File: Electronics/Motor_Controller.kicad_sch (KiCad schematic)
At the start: 43 parts, among them J2 SWCLK SWD, SW1 SW_Push, SW2 ~{USB_BOOT}, U1 RP2040, U4 W25Q32JVZP, Y1 ABM8-272-T3

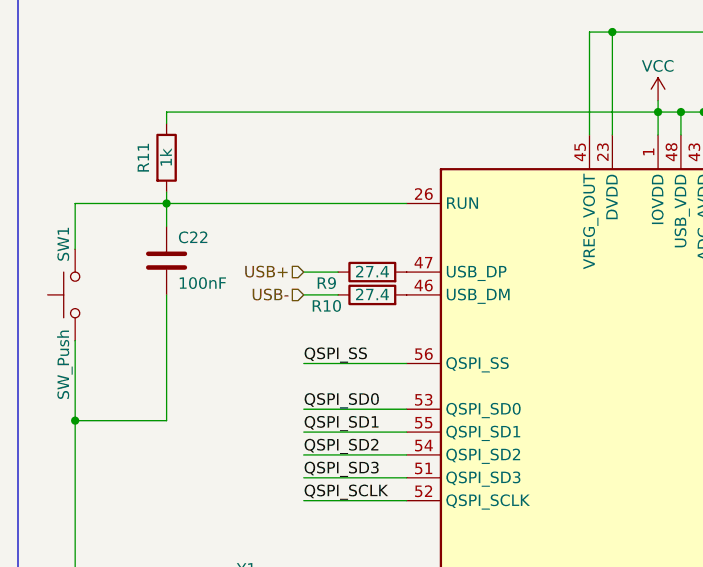
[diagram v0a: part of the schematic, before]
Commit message: power + usb
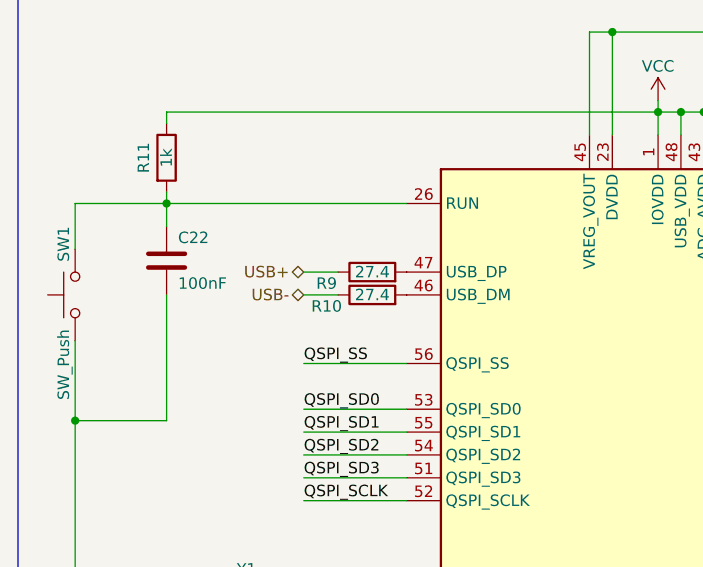
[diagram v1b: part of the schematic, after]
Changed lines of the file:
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@@
     (effects (font (size 1.27 1.27)) (justify left))
   )
-  (hierarchical_label "USB+" (shape input) (at 44.45 49.53 180) (fields_autoplaced)
+  (hierarchical_label "USB+" (shape bidirectional) (at 44.45 49.53 180) (fields_autoplaced)
     (effects (font (size 1.27 1.27)) (justify right))
   )
-  (hierarchical_label "USB-" (shape input) (at 44.45 52.07 180) (fields_autoplaced)
+  (hierarchical_label "USB-" (shape bidirectional) (at 44.45 52.07 180) (fields_autoplaced)
     (effects (font (size 1.27 1.27)) (justify right))
   )
